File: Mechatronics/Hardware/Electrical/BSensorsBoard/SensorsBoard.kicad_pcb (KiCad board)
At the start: 2 copper layers, 24 x 13.7 mm, 5 parts, among them J1 Conn_01x01_Male, J2 Conn_01x01_Male, J3 Conn_01x01_Male, J4 Conn_01x01_Male, U1 ITR1802

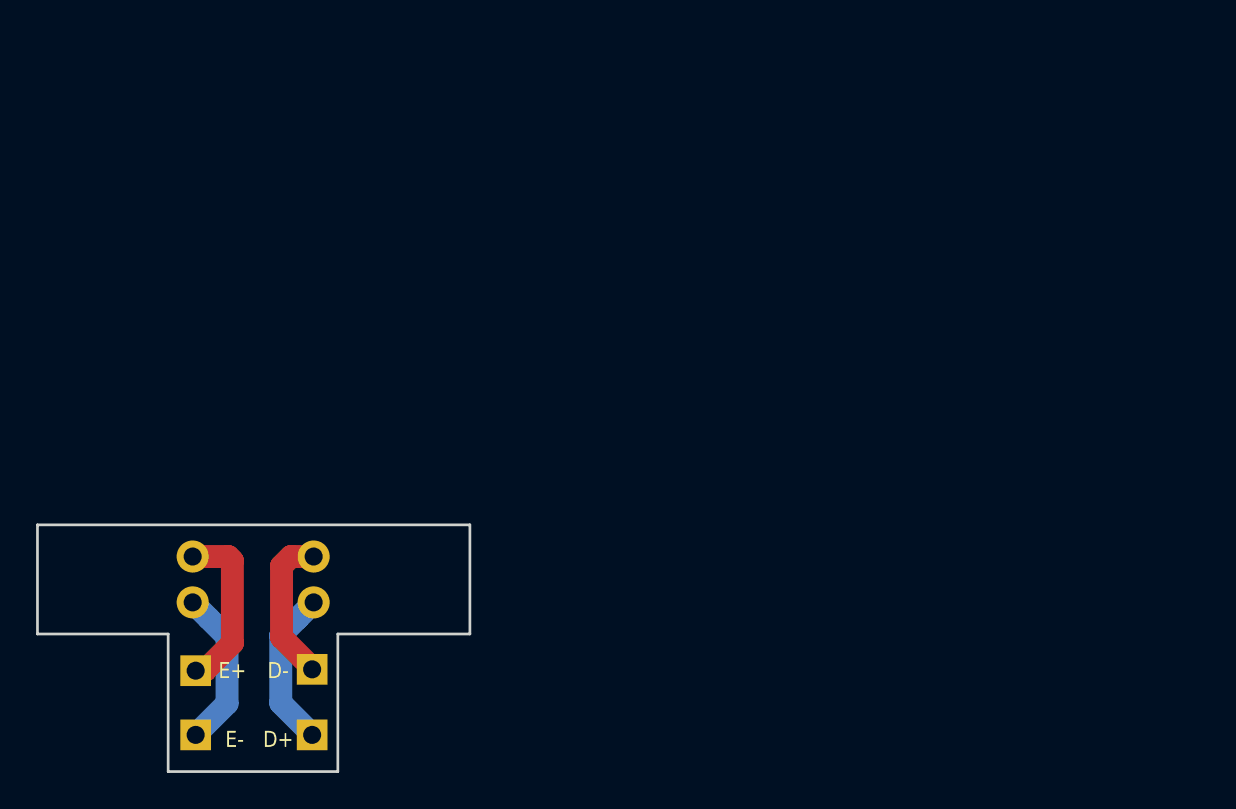
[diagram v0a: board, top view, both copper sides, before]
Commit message: Changes
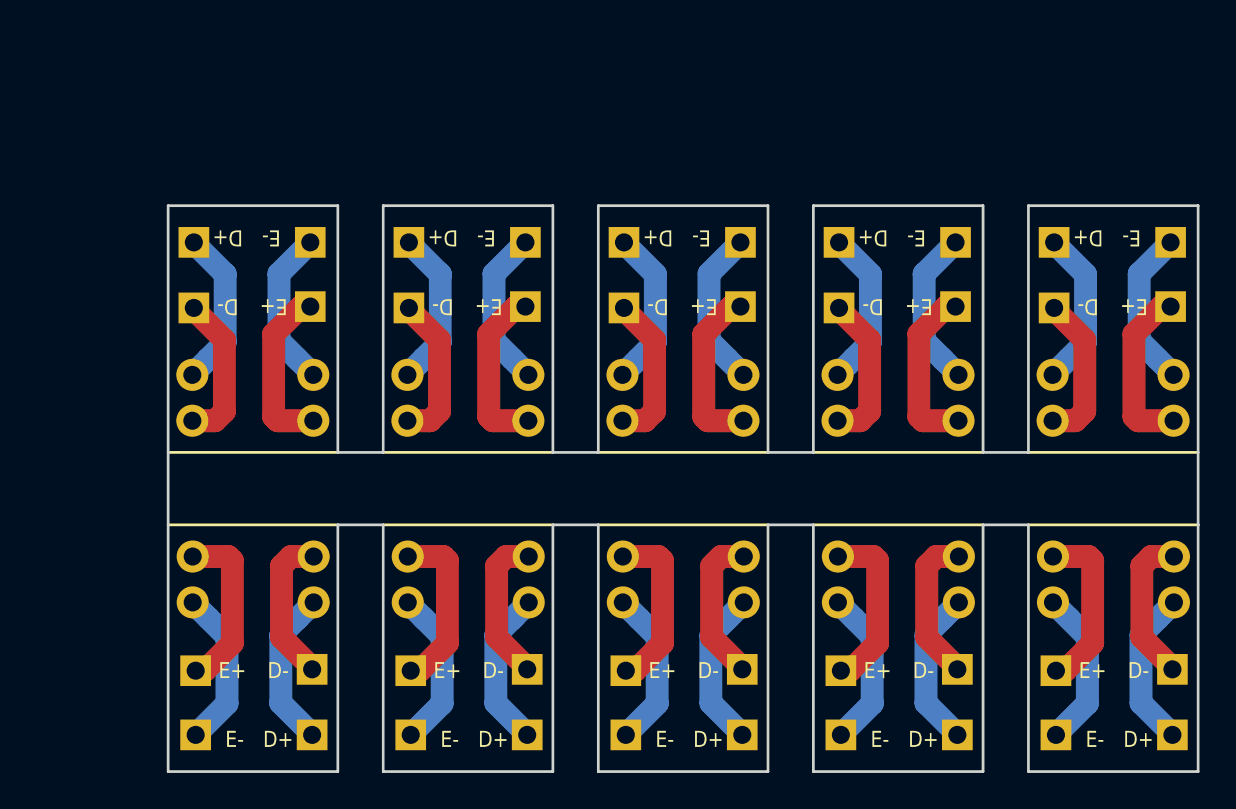
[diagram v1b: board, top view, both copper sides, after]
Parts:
- added J1: Conn_01x01_Male, Encoder:No3dmodelPinHeader_1x01_P2.54mm_Vertical, F.Cu at (222.3, 120.2)
- added J1: Conn_01x01_Male, Encoder:No3dmodelPinHeader_1x01_P2.54mm_Vertical, F.Cu at (228.7, 100.0)
- added J1: Conn_01x01_Male, Encoder:No3dmodelPinHeader_1x01_P2.54mm_Vertical, F.Cu at (210.4, 120.2)
- added J1: Conn_01x01_Male, Encoder:No3dmodelPinHeader_1x01_P2.54mm_Vertical, F.Cu at (216.7, 100.0)
- added J1: Conn_01x01_Male, Encoder:No3dmodelPinHeader_1x01_P2.54mm_Vertical, F.Cu at (198.5, 120.2)
- added J1: Conn_01x01_Male, Encoder:No3dmodelPinHeader_1x01_P2.54mm_Vertical, F.Cu at (204.8, 100.0)
- added J1: Conn_01x01_Male, Encoder:No3dmodelPinHeader_1x01_P2.54mm_Vertical, F.Cu at (186.6, 120.2)
- added J1: Conn_01x01_Male, Encoder:No3dmodelPinHeader_1x01_P2.54mm_Vertical, F.Cu at (192.9, 100.0)
- added J1: Conn_01x01_Male, Encoder:No3dmodelPinHeader_1x01_P2.54mm_Vertical, F.Cu at (181.0, 100.0)
- added J2: Conn_01x01_Male, Encoder:No3dmodelPinHeader_1x01_P2.54mm_Vertical, F.Cu at (228.7, 96.5)
- added J2: Conn_01x01_Male, Encoder:No3dmodelPinHeader_1x01_P2.54mm_Vertical, F.Cu at (222.3, 123.7)
- added J2: Conn_01x01_Male, Encoder:No3dmodelPinHeader_1x01_P2.54mm_Vertical, F.Cu at (216.7, 96.5)
- added J2: Conn_01x01_Male, Encoder:No3dmodelPinHeader_1x01_P2.54mm_Vertical, F.Cu at (210.4, 123.7)
- added J2: Conn_01x01_Male, Encoder:No3dmodelPinHeader_1x01_P2.54mm_Vertical, F.Cu at (204.8, 96.5)
- added J2: Conn_01x01_Male, Encoder:No3dmodelPinHeader_1x01_P2.54mm_Vertical, F.Cu at (198.5, 123.7)
- added J2: Conn_01x01_Male, Encoder:No3dmodelPinHeader_1x01_P2.54mm_Vertical, F.Cu at (186.6, 123.7)
- added J2: Conn_01x01_Male, Encoder:No3dmodelPinHeader_1x01_P2.54mm_Vertical, F.Cu at (192.9, 96.5)
- added J2: Conn_01x01_Male, Encoder:No3dmodelPinHeader_1x01_P2.54mm_Vertical, F.Cu at (181.0, 96.5)
- added J3: Conn_01x01_Male, Encoder:No3dmodelPinHeader_1x01_P2.54mm_Vertical, F.Cu at (222.2, 100.1)
- added J3: Conn_01x01_Male, Encoder:No3dmodelPinHeader_1x01_P2.54mm_Vertical, F.Cu at (228.8, 120.1)
- added J3: Conn_01x01_Male, Encoder:No3dmodelPinHeader_1x01_P2.54mm_Vertical, F.Cu at (210.3, 100.1)
- added J3: Conn_01x01_Male, Encoder:No3dmodelPinHeader_1x01_P2.54mm_Vertical, F.Cu at (216.8, 120.1)
- added J3: Conn_01x01_Male, Encoder:No3dmodelPinHeader_1x01_P2.54mm_Vertical, F.Cu at (198.4, 100.1)
- added J3: Conn_01x01_Male, Encoder:No3dmodelPinHeader_1x01_P2.54mm_Vertical, F.Cu at (204.9, 120.1)
- added J3: Conn_01x01_Male, Encoder:No3dmodelPinHeader_1x01_P2.54mm_Vertical, F.Cu at (186.5, 100.1)
- added J3: Conn_01x01_Male, Encoder:No3dmodelPinHeader_1x01_P2.54mm_Vertical, F.Cu at (193.0, 120.1)
- added J3: Conn_01x01_Male, Encoder:No3dmodelPinHeader_1x01_P2.54mm_Vertical, F.Cu at (174.5, 100.1)
- added J4: Conn_01x01_Male, Encoder:No3dmodelPinHeader_1x01_P2.54mm_Vertical, F.Cu at (228.8, 123.7)
- added J4: Conn_01x01_Male, Encoder:No3dmodelPinHeader_1x01_P2.54mm_Vertical, F.Cu at (222.2, 96.5)
- added J4: Conn_01x01_Male, Encoder:No3dmodelPinHeader_1x01_P2.54mm_Vertical, F.Cu at (216.8, 123.7)
- added J4: Conn_01x01_Male, Encoder:No3dmodelPinHeader_1x01_P2.54mm_Vertical, F.Cu at (210.3, 96.5)
- added J4: Conn_01x01_Male, Encoder:No3dmodelPinHeader_1x01_P2.54mm_Vertical, F.Cu at (204.9, 123.7)
- added J4: Conn_01x01_Male, Encoder:No3dmodelPinHeader_1x01_P2.54mm_Vertical, F.Cu at (198.4, 96.5)
- added J4: Conn_01x01_Male, Encoder:No3dmodelPinHeader_1x01_P2.54mm_Vertical, F.Cu at (186.5, 96.5)
- added J4: Conn_01x01_Male, Encoder:No3dmodelPinHeader_1x01_P2.54mm_Vertical, F.Cu at (193.0, 123.7)
- added J4: Conn_01x01_Male, Encoder:No3dmodelPinHeader_1x01_P2.54mm_Vertical, F.Cu at (174.5, 96.5)
- added U1: ITR1802, Encoder:itr8102, F.Cu at (225.5, 115.1)
- added U1: ITR1802, Encoder:itr8102, F.Cu at (225.5, 105.1)
- added U1: ITR1802, Encoder:itr8102, F.Cu at (213.6, 115.1)
- added U1: ITR1802, Encoder:itr8102, F.Cu at (213.6, 105.1)
- added U1: ITR1802, Encoder:itr8102, F.Cu at (201.7, 115.1)
- added U1: ITR1802, Encoder:itr8102, F.Cu at (201.6, 105.1)
- added U1: ITR1802, Encoder:itr8102, F.Cu at (189.7, 105.1)
- added U1: ITR1802, Encoder:itr8102, F.Cu at (189.7, 115.1)
- added U1: ITR1802, Encoder:itr8102, F.Cu at (177.8, 105.1)
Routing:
- net (no net): track 35.6 -> 356.1 mm
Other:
- board size 24 x 13.7 mm -> 57 x 31.3 mm

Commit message: Changes
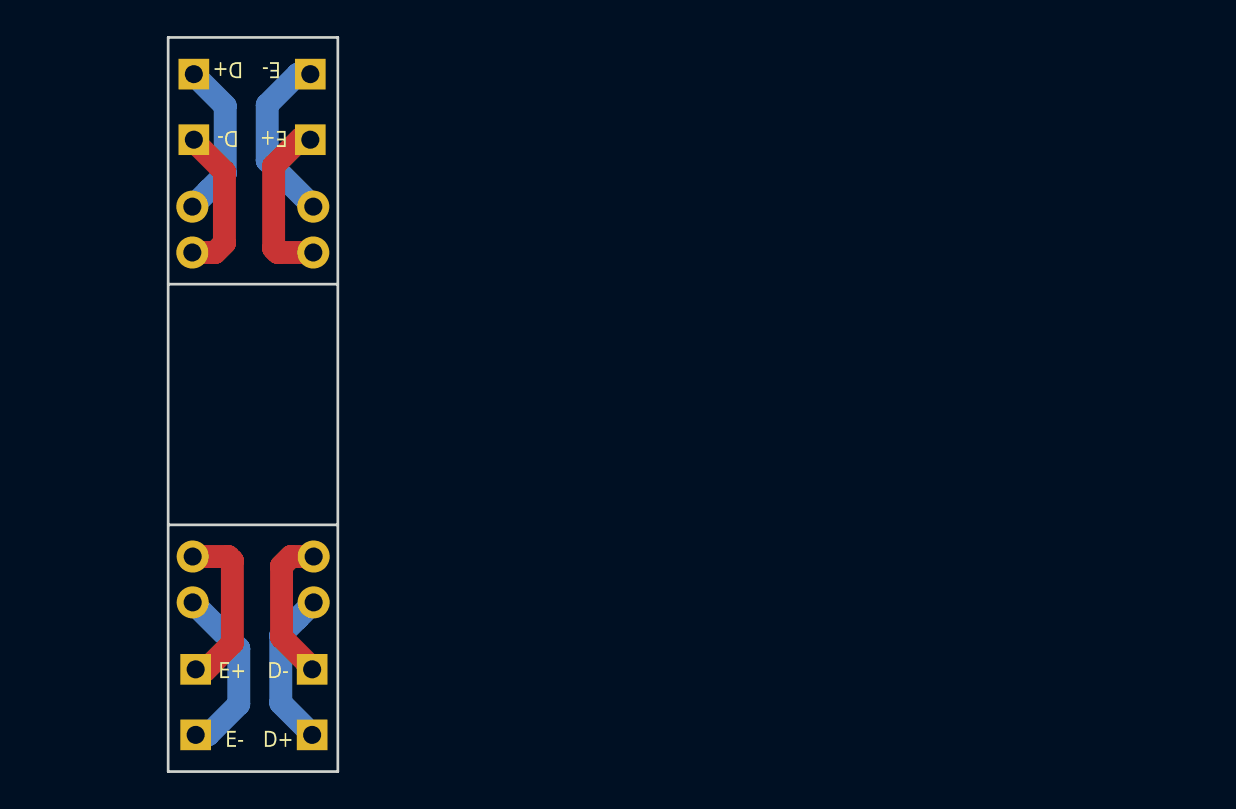
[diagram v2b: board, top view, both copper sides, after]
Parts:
- removed the J1 at (222.3, 120.2)
- removed the J1 at (228.7, 100.0)
- removed the J1 at (210.4, 120.2)
- removed the J1 at (216.7, 100.0)
- removed the J1 at (198.5, 120.2)
- removed the J1 at (204.8, 100.0)
- removed the J1 at (186.6, 120.2)
- removed the J1 at (192.9, 100.0)
- removed the J1 at (181.0, 100.0)
- removed the J2 at (228.7, 96.5)
- removed the J2 at (222.3, 123.7)
- removed the J2 at (216.7, 96.5)
- removed the J2 at (210.4, 123.7)
- removed the J2 at (204.8, 96.5)
- removed the J2 at (198.5, 123.7)
- removed the J2 at (186.6, 123.7)
- removed the J2 at (192.9, 96.5)
- removed the J2 at (181.0, 96.5)
- removed the J3 at (222.2, 100.1)
- removed the J3 at (228.8, 120.1)
- removed the J3 at (210.3, 100.1)
- removed the J3 at (216.8, 120.1)
- removed the J3 at (198.4, 100.1)
- removed the J3 at (204.9, 120.1)
- removed the J3 at (186.5, 100.1)
- removed the J3 at (193.0, 120.1)
- removed the J3 at (174.5, 100.1)
- removed the J4 at (228.8, 123.7)
- removed the J4 at (222.2, 96.5)
- removed the J4 at (216.8, 123.7)
- removed the J4 at (210.3, 96.5)
- removed the J4 at (204.9, 123.7)
- removed the J4 at (198.4, 96.5)
- removed the J4 at (186.5, 96.5)
- removed the J4 at (193.0, 123.7)
- removed the J4 at (174.5, 96.5)
- removed the U1 at (225.5, 115.1)
- removed the U1 at (225.5, 105.1)
- removed the U1 at (213.6, 115.1)
- removed the U1 at (213.6, 105.1)
- removed the U1 at (201.7, 115.1)
- removed the U1 at (201.6, 105.1)
- removed the U1 at (189.7, 105.1)
- removed the U1 at (189.7, 115.1)
- removed the U1 at (177.8, 105.1)
- added J1: Conn_01x01_Male, Encoder:No3dmodelPinHeader_1x01_P2.54mm_Vertical, F.Cu at (181.0, 90.8)
- added J2: Conn_01x01_Male, Encoder:No3dmodelPinHeader_1x01_P2.54mm_Vertical, F.Cu at (181.0, 87.2)
- added J3: Conn_01x01_Male, Encoder:No3dmodelPinHeader_1x01_P2.54mm_Vertical, F.Cu at (174.5, 90.8)
- added J4: Conn_01x01_Male, Encoder:No3dmodelPinHeader_1x01_P2.54mm_Vertical, F.Cu at (174.5, 87.2)
- added U1: ITR1802, Encoder:itr8102, F.Cu at (177.8, 95.8)
- moved J1 0.08 mm to (174.7, 120.1)
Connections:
- J1 pad 1: (no net) -> Net-(J1-Pad1)
- J2 pad 1: (no net) -> Net-(J2-Pad1)
- J3 pad 1: (no net) -> Net-(J3-Pad1)
- J4 pad 1: (no net) -> Net-(J4-Pad1)
- U1 pad 1: (no net) -> Net-(J1-Pad1)
- U1 pad 2: (no net) -> Net-(J2-Pad1)
- U1 pad 3: (no net) -> Net-(J4-Pad1)
- U1 pad 4: (no net) -> Net-(J3-Pad1)
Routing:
- net (no net): track 356.1 -> 36.6 mm
- net Net-(J2-Pad1): track 0.00 -> 9.79 mm
- net Net-(J1-Pad1): track 0.00 -> 9.53 mm
- net Net-(J4-Pad1): track 0.00 -> 8.81 mm
- net Net-(J3-Pad1): track 0.00 -> 8.42 mm
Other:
- board size 57 x 31.3 mm -> 9.4 x 40.7 mm
- net class Default: clearance 0.254 -> 0.127; trace_width 0.254 -> 0.127
- rule trace_clearance: 0.254 -> 0.127
- rule trace_min: 0.254 -> 0.127
